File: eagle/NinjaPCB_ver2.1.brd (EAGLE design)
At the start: 79 x 73 mm, 72 parts, among them IC1 ANALOGSW_AD_SOT23-6, IC2 NAU7802, Q1 IRLB3813PBF, Q2 CJ2302, Q3 CJ2302, Q4 S9013, Q5 S9013, Q6 S9013

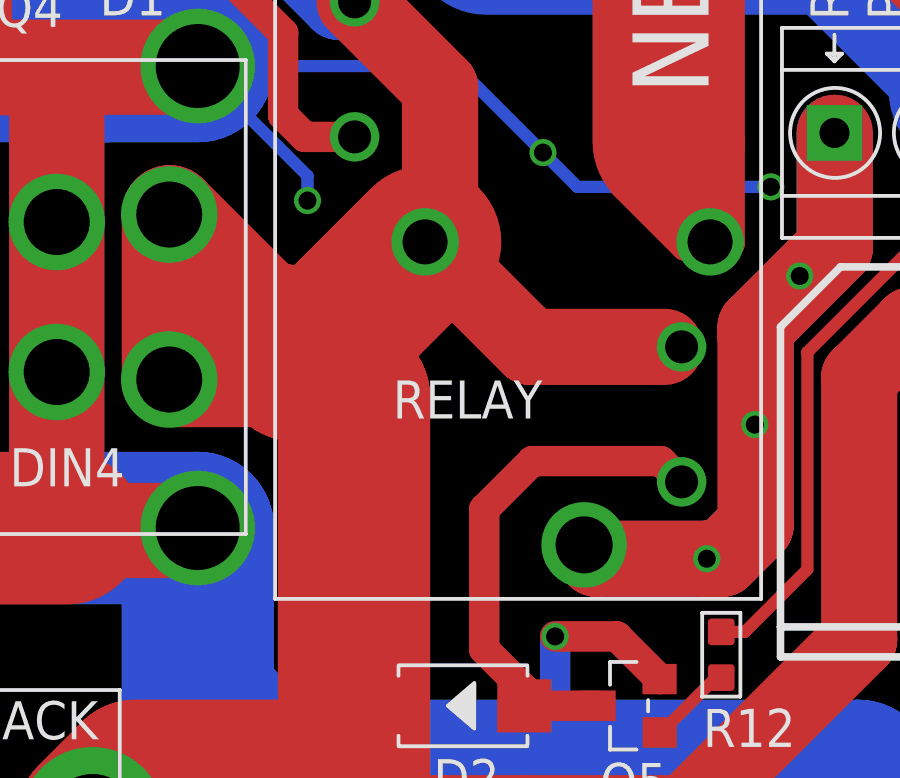
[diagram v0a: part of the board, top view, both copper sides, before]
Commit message: minor update for layout
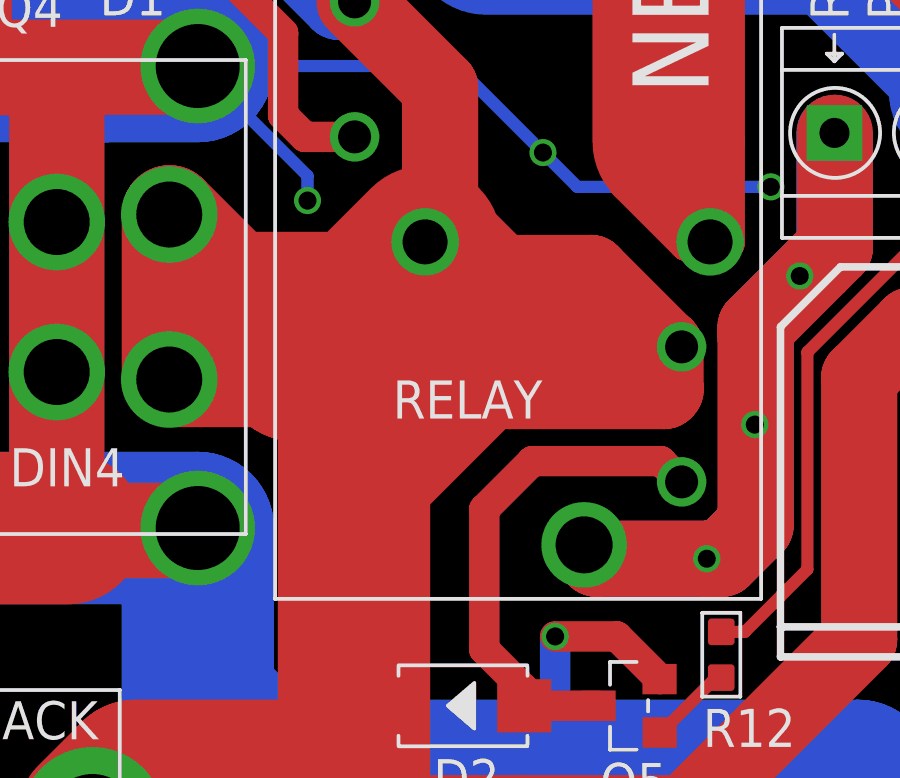
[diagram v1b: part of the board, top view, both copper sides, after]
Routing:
- net 12V: track 195.4 -> 234.3 mm

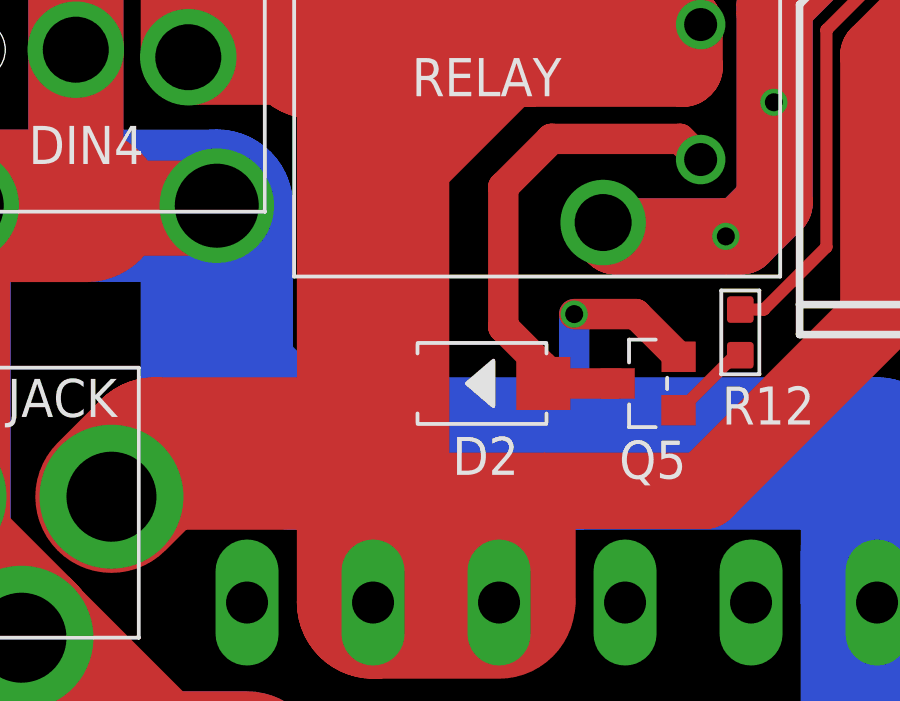
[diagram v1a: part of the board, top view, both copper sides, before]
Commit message: minor update for layout
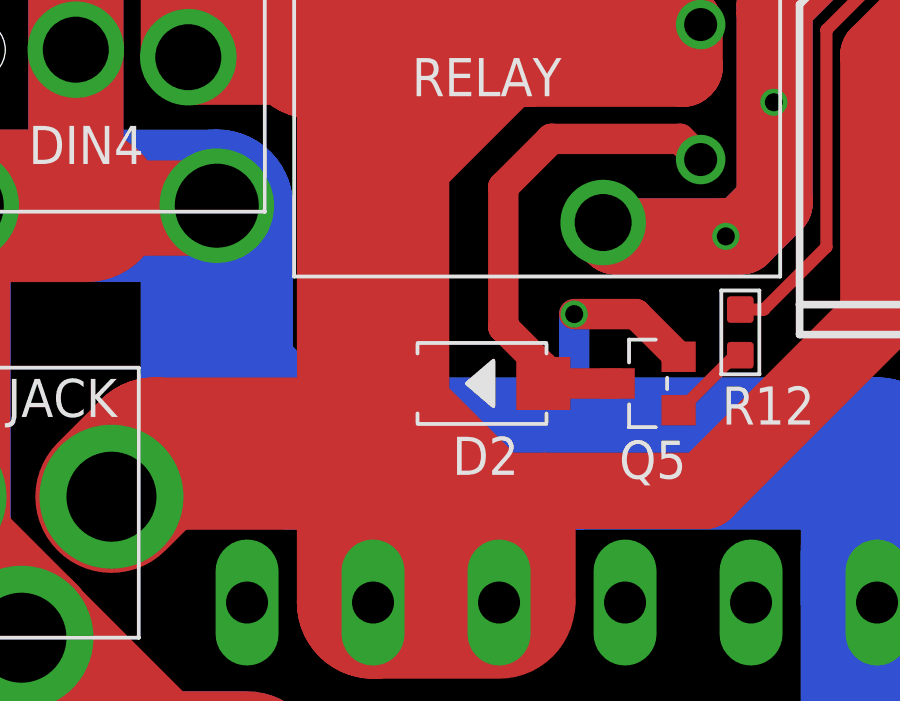
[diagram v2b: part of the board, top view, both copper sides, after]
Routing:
- net 12V: track 234.3 -> 248.3 mm
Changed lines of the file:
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@@
 <wire x1="28.372" y1="27.8386" x2="28.3591" y2="27.8386" width="0.254" layer="1"/>
 <wire x1="28.3591" y1="27.8386" x2="28.3591" y2="27.8511" width="0.254" layer="1"/>
+<wire x1="19.2532" y1="21.3868" x2="19.2532" y2="15.2146" width="2.54" layer="1"/>
+<wire x1="19.2532" y1="15.2146" x2="21.8948" y2="12.573" width="2.54" layer="1"/>
+<wire x1="19.2532" y1="15.2146" x2="20.3962" y2="15.2146" width="0.254" layer="1"/>
+<wire x1="20.3962" y1="15.2146" x2="20.3962" y2="12.2936" width="0.254" layer="1"/>
 </signal>
 <signal name="N$2">

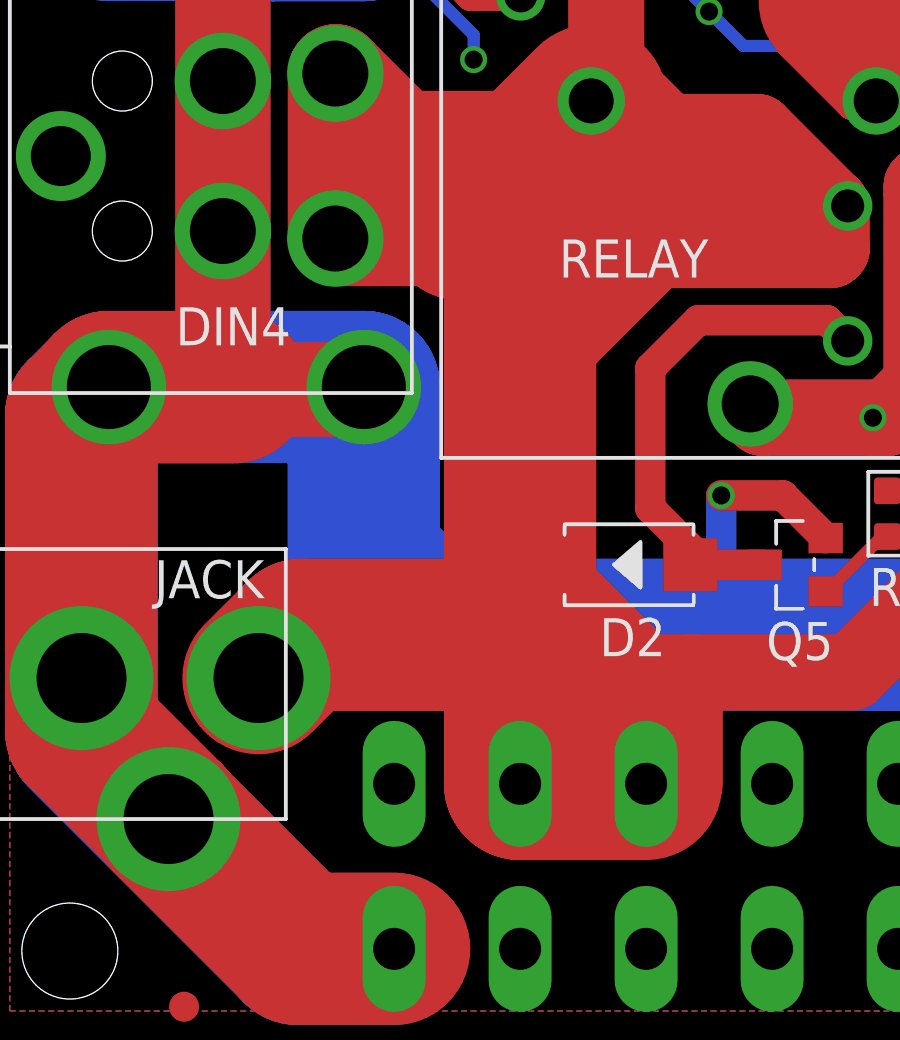
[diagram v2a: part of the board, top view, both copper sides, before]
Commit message: minor update for layout
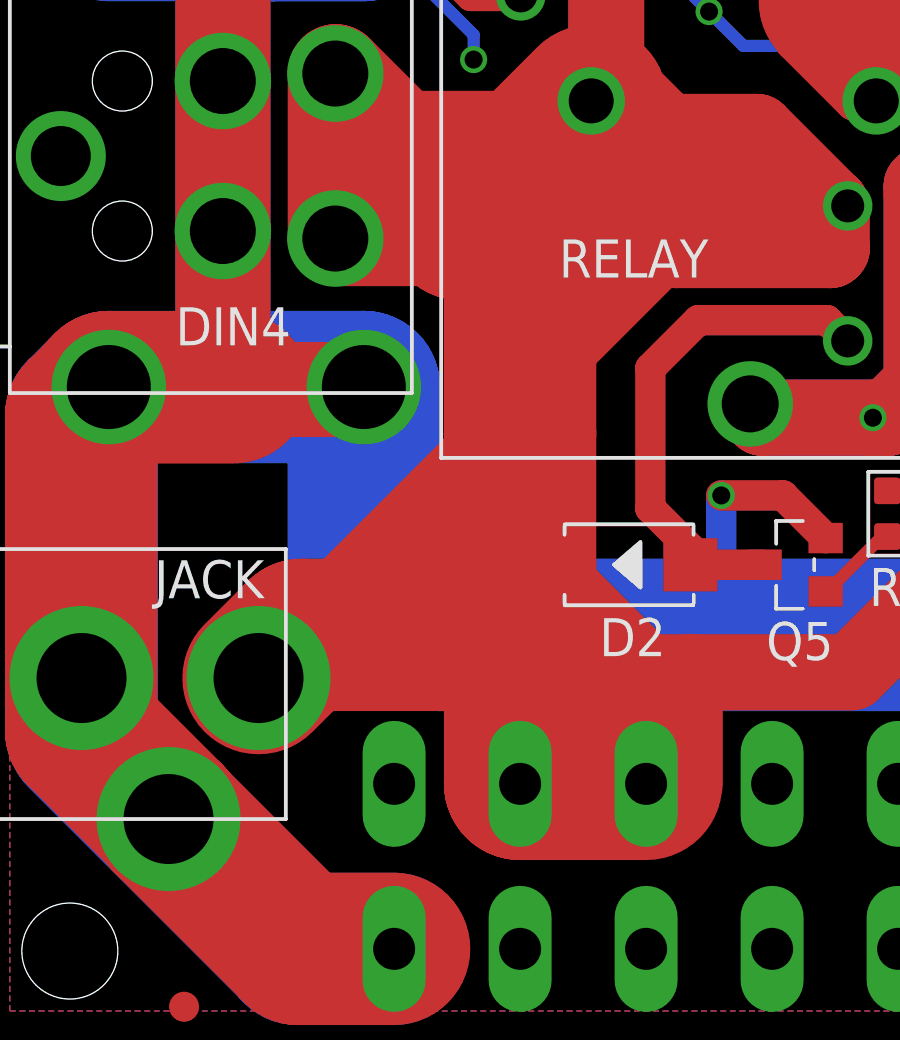
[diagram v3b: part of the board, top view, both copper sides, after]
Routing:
- net 12V: track 248.3 -> 263.8 mm
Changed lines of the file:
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@@
 <wire x1="19.7358" y1="53.8226" x2="19.7358" y2="50.3428" width="2.54" layer="16"/>
 <wire x1="16.7132" y1="27.4574" x2="18.0092" y2="26.1614" width="5.08" layer="1"/>
-<wire x1="18.0092" y1="26.1614" x2="18.0092" y2="8.5726" width="5.08" layer="1"/>
+<wire x1="18.0092" y1="26.1614" x2="18.0092" y2="20.2438" width="5.08" layer="1"/>
+<wire x1="18.0092" y1="20.2438" x2="18.0092" y2="8.5726" width="5.08" layer="1"/>
 <wire x1="9.29" y1="12.1" x2="10.7282" y2="13.5382" width="5.08" layer="1"/>
 <wire x1="10.7282" y1="13.5382" x2="17.3228" y2="13.5382" width="5.08" layer="1"/>
@@
 <wire x1="19.2532" y1="15.2146" x2="20.3962" y2="15.2146" width="0.254" layer="1"/>
 <wire x1="20.3962" y1="15.2146" x2="20.3962" y2="12.2936" width="0.254" layer="1"/>
+<wire x1="17.1958" y1="23.2664" x2="17.1958" y2="20.0152" width="2.54" layer="1"/>
+<wire x1="17.1958" y1="20.0152" x2="12.065" y2="14.8844" width="2.54" layer="1"/>
+<wire x1="12.065" y1="14.8844" x2="14.5542" y2="14.8844" width="2.54" layer="1"/>
+<wire x1="14.5542" y1="14.8844" x2="15.5956" y2="15.9258" width="2.54" layer="1"/>
+<wire x1="17.1958" y1="20.0152" x2="18.0092" y2="20.0152" width="0.254" layer="1"/>
+<wire x1="18.0092" y1="20.0152" x2="18.0092" y2="20.2438" width="0.254" layer="1"/>
 </signal>
 <signal name="N$2">
